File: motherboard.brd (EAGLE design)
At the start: 177.1 x 75.9 mm, 187 parts, among them IC1 LM2576, IC10 TUSB2046B, IC12 LM50, IC13 LM50, IC2 74LS595D, IC3 74LS595D, IC4 IC_FT230X-SSOP-16, IC5 VN5772AK, IC6 VN5772AK, IC7 VN5772AK, IC8 VN5772AK, IC9 VN5772AK, U2 NCP4625, U3 ATMEGA168, Y1 16Mhz, Y2 6MHz

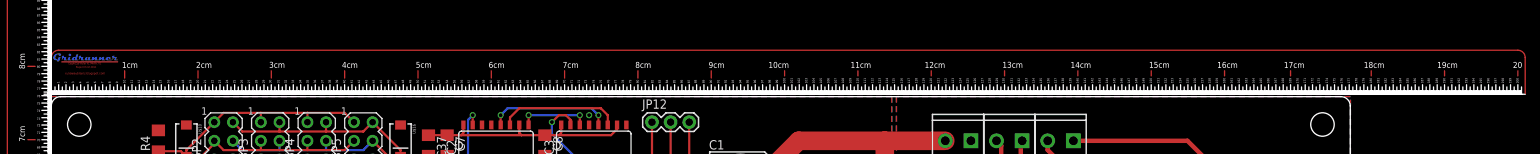
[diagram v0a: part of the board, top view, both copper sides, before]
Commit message: moved ruler
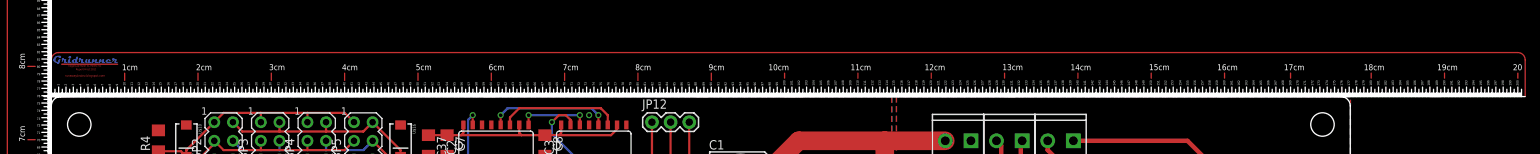
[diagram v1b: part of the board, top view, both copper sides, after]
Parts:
- moved U$17 0.32 mm to (0.00, 75.9)
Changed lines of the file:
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@@
 <?xml version="1.0" encoding="utf-8"?>
 <!DOCTYPE eagle SYSTEM "eagle.dtd">
-<eagle version="6.5.0">
+<eagle version="6.1">
 <drawing>
 <settings>
@@
 </class>
 </classes>
-<designrules name="default">
+<designrules>
 <description language="de">&lt;b&gt;EAGLE Design Rules&lt;/b&gt;
 &lt;p&gt;
@@
 <element name="D5" library="adafruit" package="SOD-123" value="" x="143.51" y="15.24" rot="R180"/>
 <element name="SW1" library="alcoswitch" package="FSMSM" value="" x="-37.465" y="46.355"/>
-<element name="U$17" library="CAD Ruler_EagleCad Gridrunner XL Metric V1 (Rupert Hirst 2011)" package="RULER" value="" x="0" y="76.2"/>
+<element name="U$17" library="CAD Ruler_EagleCad Gridrunner XL Metric V1 (Rupert Hirst 2011)" package="RULER" value="" x="0" y="75.8825"/>
 <element name="U$18" library="CAD Ruler_EagleCad Gridrunner XL Metric V1 (Rupert Hirst 2011)" package="RULER" value="" x="0" y="0" rot="R90"/>
 <element name="C43" library="adafruit" package="C1206" value="0.1uF" x="30.48" y="7.62"/>
